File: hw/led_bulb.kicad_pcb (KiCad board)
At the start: 2 copper layers, 136 x 50 mm, 181 parts, among them P1 USB_OTG, P10 CONN_01X04, P11 CONN_01X04, P12 CONN_01X04, P13 CONN_01X04, P14 CONN_01X04, P15 CONN_01X04, P16 CONN_01X04, P17 CONN_01X04, P2 CONN_01X04, P3 CONN_01X04, P4 CONN_01X04, P5 CONN_01X04, P6 CONN_01X04, P7 CONN_01X04, P8 CONN_01X04, P9 CONN_01X04, SW1 SW_RST, SW2 SW_FLASH, U1 CP2102, U3 ESP-12E, U4 AP1117D33

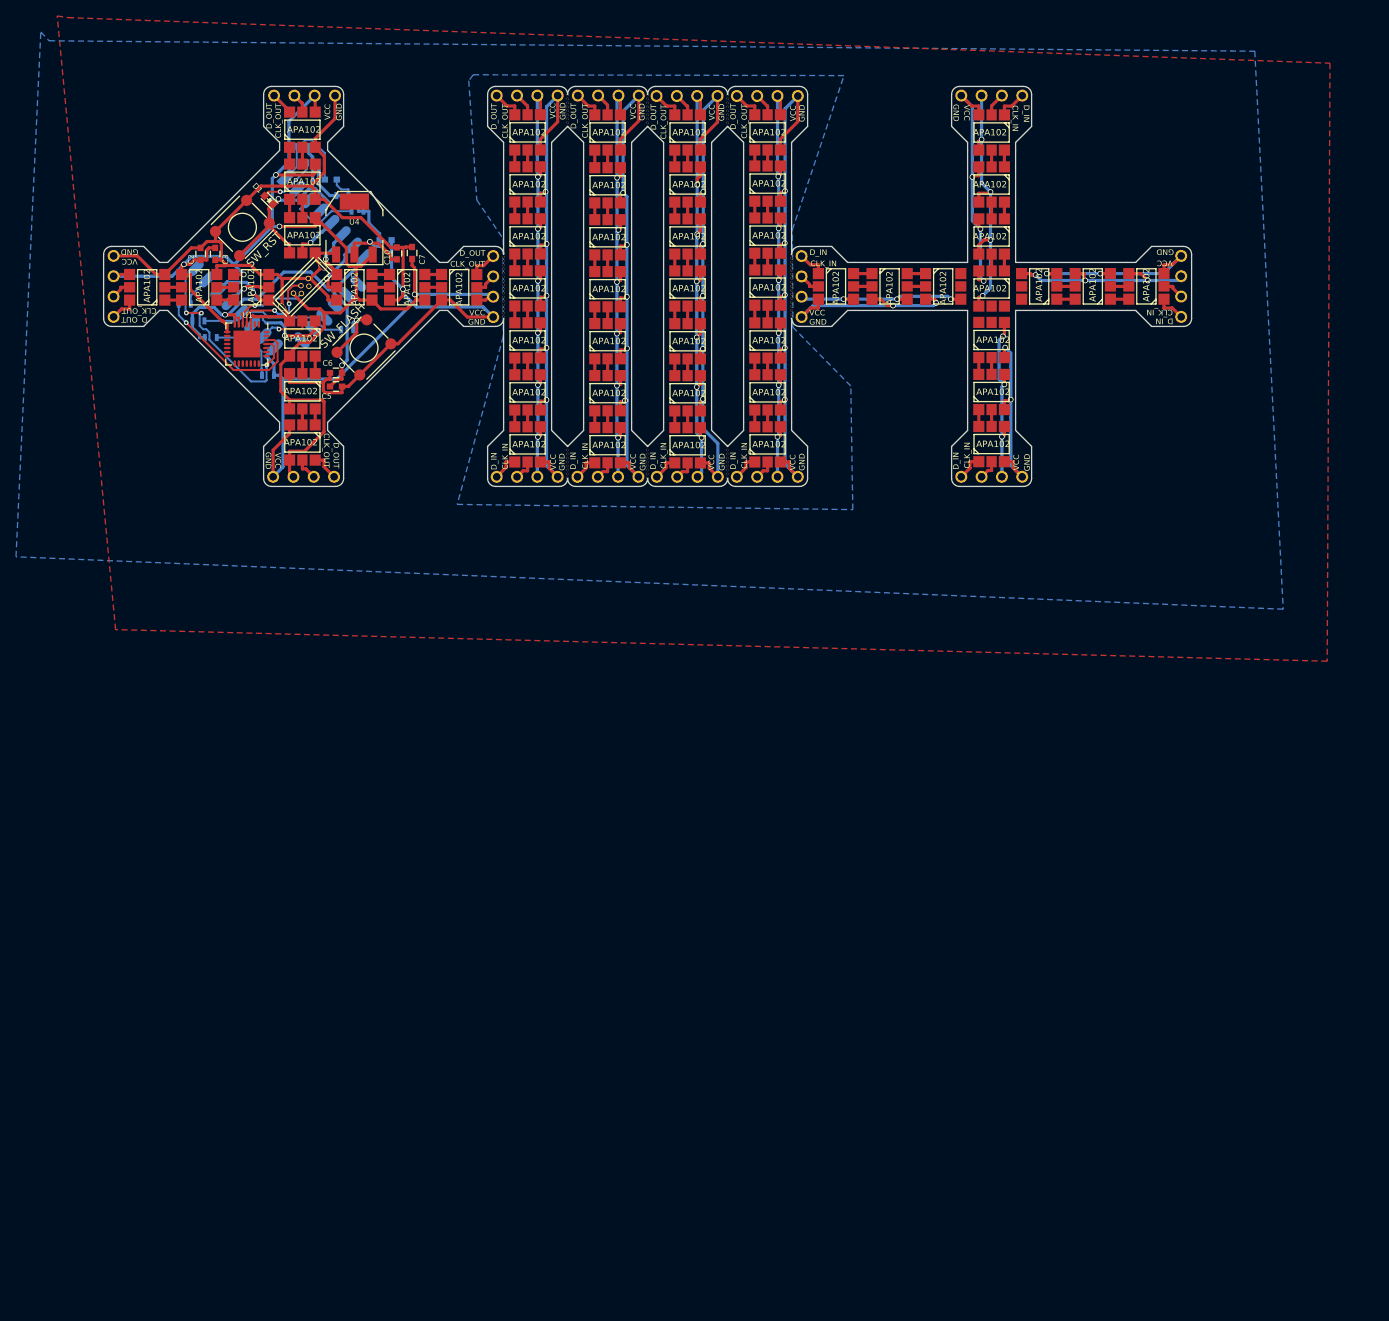
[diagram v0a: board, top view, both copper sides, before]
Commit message: Added first version of v4 hardware.
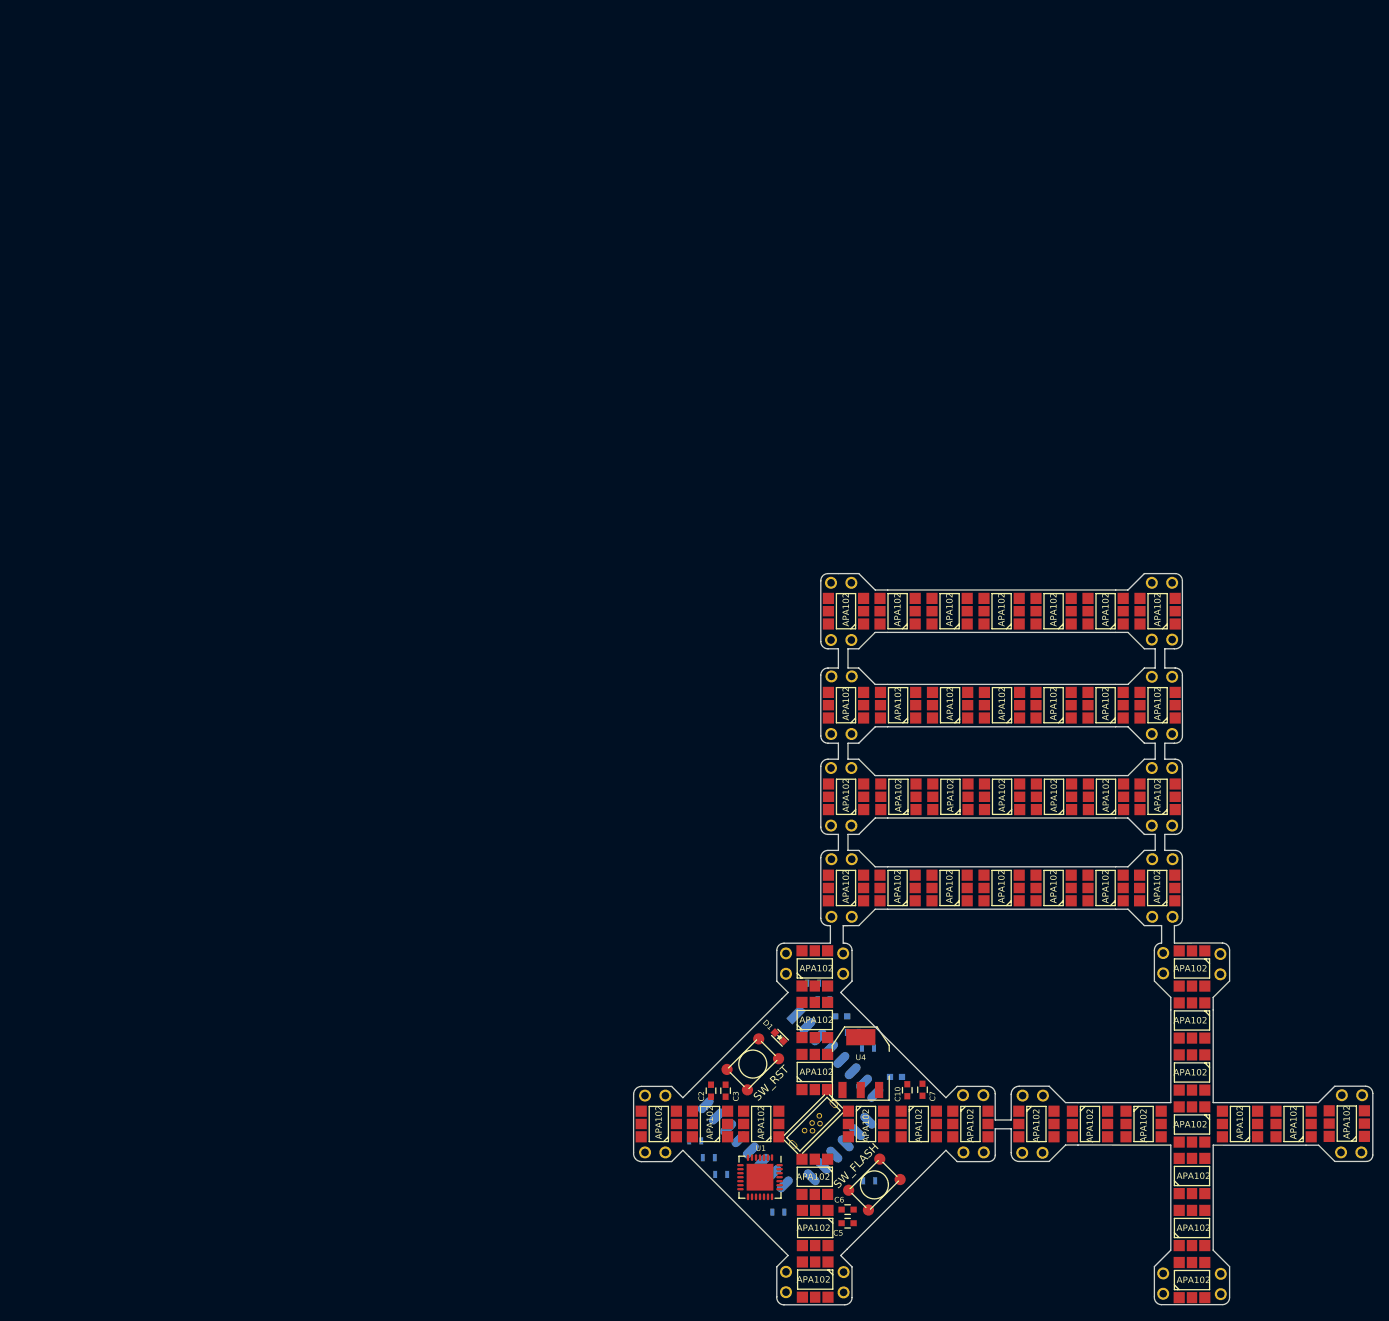
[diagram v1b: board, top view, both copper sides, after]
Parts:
- removed HOLE0 (x88): 0.3mm, footprints:0.3mm
- added P18: CONN_01X02, footprints:CONN_2.54mm_1x2_no-outline, F.Cu at (156.4, 125.6)
- added P19: CONN_01X02, footprints:CONN_2.54mm_1x2_no-outline, F.Cu at (149.2, 125.5)
- added P20: CONN_01X02, footprints:CONN_2.54mm_1x2_no-outline, F.Cu at (172.8, 149.2)
- added P21: CONN_01X02, footprints:CONN_2.54mm_1x2_no-outline, F.Cu at (172.8, 142.0)
- added P22: CONN_01X02, footprints:CONN_2.54mm_1x2_no-outline, F.Cu at (149.2, 165.6)
- added P23: CONN_01X02, footprints:CONN_2.54mm_1x2_no-outline, F.Cu at (156.4, 165.6)
- added P24: CONN_01X02, footprints:CONN_2.54mm_1x2_no-outline, F.Cu at (132.9, 142.1)
- added P25: CONN_01X02, footprints:CONN_2.54mm_1x2_no-outline, F.Cu at (132.9, 149.2)
- added P26: CONN_01X02, footprints:CONN_2.54mm_1x2_no-outline, F.Cu at (109.0, 85.1)
- added P27: CONN_01X02, footprints:CONN_2.54mm_1x2_no-outline, F.Cu at (109.0, 78.0)
- added P28: CONN_01X02, footprints:CONN_2.54mm_1x2_no-outline, F.Cu at (109.0, 96.8)
- added P29: CONN_01X02, footprints:CONN_2.54mm_1x2_no-outline, F.Cu at (109.0, 89.7)
- added P30: CONN_01X02, footprints:CONN_2.54mm_1x2_no-outline, F.Cu at (109.0, 108.3)
- added P31: CONN_01X02, footprints:CONN_2.54mm_1x2_no-outline, F.Cu at (109.0, 101.1)
- added P32: CONN_01X02, footprints:CONN_2.54mm_1x2_no-outline, F.Cu at (109.0, 119.7)
- added P33: CONN_01X02, footprints:CONN_2.54mm_1x2_no-outline, F.Cu at (109.0, 112.5)
- P10, P11, P12, P13, P14, P15, P16, P17, P2, P3, P4, P5, P6, P7, P8, P9: value CONN_01X04 -> CONN_01X02; footprint footprints:CONN_2.54mm_1x4_no-outline -> footprints:CONN_2.54mm_1x2_no-outline
- SW1, SW2: footprint footprints:switch_spst_smd_5.5mm_4.5mm -> footprints:switch_spst_smd_5mm_3.5mm
- moved P5 150.2 mm to (102.1, 165.3), turned to 90 degrees
- moved R9 124.8 mm to (112.5, 152.7)
- moved P2 124.1 mm to (102.1, 125.5), turned to 270 degrees
- moved LED9 122.9 mm to (105.7, 126.2)
- moved LED3 122.8 mm to (105.7, 152.2)
- moved LED5 122.8 mm to (105.7, 132.6)
- moved LED11 122.7 mm to (105.8, 165.1)
- moved LED7 122.7 mm to (105.8, 158.6)
- moved LED1 122.6 mm to (105.7, 139.1)
- moved P1 122.6 mm to (103.8, 149.0)
- moved LED12 122.6 mm to (86.2, 145.6)
- moved LED6 122.6 mm to (118.7, 145.6)
- moved C5 122.6 mm to (109.8, 158.0)
- moved C6 122.6 mm to (109.8, 156.3)
- moved LED2 122.6 mm to (112.1, 145.6)
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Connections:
- net DTR renamed Net-(U1-Pad28)
- net RTS renamed Net-(U1-Pad24)
- LED1 pad 1: GPIO16 -> GPIO0
- LED13 pad 3: GND -> Net-(LED13-Pad3)
- LED13 pad 4: V_USB -> Net-(LED13-Pad4)
- LED14 pad 3: GND -> Net-(LED14-Pad3)
- LED14 pad 4: V_USB -> Net-(LED14-Pad4)
- LED15 pad 3: GND -> Net-(LED15-Pad3)
- LED15 pad 4: V_USB -> Net-(LED15-Pad4)
- LED16 pad 3: GND -> Net-(LED16-Pad3)
- LED16 pad 4: V_USB -> Net-(LED16-Pad4)
- LED17 pad 3: GND -> Net-(LED13-Pad3)
- LED17 pad 4: V_USB -> Net-(LED13-Pad4)
- LED18 pad 3: GND -> Net-(LED14-Pad3)
- LED18 pad 4: V_USB -> Net-(LED14-Pad4)
- LED19 pad 3: GND -> Net-(LED15-Pad3)
- LED19 pad 4: V_USB -> Net-(LED15-Pad4)
- LED20 pad 3: GND -> Net-(LED16-Pad3)
- LED20 pad 4: V_USB -> Net-(LED16-Pad4)
- LED21 pad 3: GND -> Net-(LED13-Pad3)
- LED21 pad 4: V_USB -> Net-(LED13-Pad4)
- LED22 pad 3: GND -> Net-(LED14-Pad3)
- LED22 pad 4: V_USB -> Net-(LED14-Pad4)
- LED23 pad 3: GND -> Net-(LED15-Pad3)
- LED23 pad 4: V_USB -> Net-(LED15-Pad4)
- LED24 pad 3: GND -> Net-(LED16-Pad3)
- LED24 pad 4: V_USB -> Net-(LED16-Pad4)
- LED25 pad 3: GND -> Net-(LED13-Pad3)
- LED25 pad 4: V_USB -> Net-(LED13-Pad4)
- LED26 pad 3: GND -> Net-(LED14-Pad3)
- LED26 pad 4: V_USB -> Net-(LED14-Pad4)
- LED27 pad 3: GND -> Net-(LED15-Pad3)
- LED27 pad 4: V_USB -> Net-(LED15-Pad4)
- LED28 pad 3: GND -> Net-(LED16-Pad3)
- LED28 pad 4: V_USB -> Net-(LED16-Pad4)
- LED29 pad 3: GND -> Net-(LED13-Pad3)
- LED29 pad 4: V_USB -> Net-(LED13-Pad4)
- LED30 pad 3: GND -> Net-(LED14-Pad3)
- LED30 pad 4: V_USB -> Net-(LED14-Pad4)
- LED31 pad 3: GND -> Net-(LED15-Pad3)
- LED31 pad 4: V_USB -> Net-(LED15-Pad4)
- LED32 pad 3: GND -> Net-(LED16-Pad3)
- LED32 pad 4: V_USB -> Net-(LED16-Pad4)
- LED33 pad 3: GND -> Net-(LED13-Pad3)
- LED33 pad 4: V_USB -> Net-(LED13-Pad4)
- LED34 pad 3: GND -> Net-(LED14-Pad3)
- LED34 pad 4: V_USB -> Net-(LED14-Pad4)
- LED35 pad 3: GND -> Net-(LED15-Pad3)
- LED35 pad 4: V_USB -> Net-(LED15-Pad4)
- LED36 pad 3: GND -> Net-(LED16-Pad3)
- LED36 pad 4: V_USB -> Net-(LED16-Pad4)
- LED37 pad 3: GND -> Net-(LED13-Pad3)
- LED37 pad 4: V_USB -> Net-(LED13-Pad4)
- LED38 pad 3: GND -> Net-(LED14-Pad3)
- LED38 pad 4: V_USB -> Net-(LED14-Pad4)
- LED39 pad 3: GND -> Net-(LED15-Pad3)
- LED39 pad 4: V_USB -> Net-(LED15-Pad4)
- LED40 pad 3: GND -> Net-(LED16-Pad3)
- LED40 pad 4: V_USB -> Net-(LED16-Pad4)
- LED41 pad 3: GND -> Net-(LED41-Pad3)
- LED41 pad 4: V_USB -> Net-(LED41-Pad4)
- LED42 pad 3: GND -> Net-(LED42-Pad3)
- LED42 pad 4: V_USB -> Net-(LED42-Pad4)
- LED43 pad 3: GND -> Net-(LED43-Pad3)
- LED43 pad 4: V_USB -> Net-(LED43-Pad4)
- LED44 pad 3: GND -> Net-(LED44-Pad3)
- LED44 pad 4: V_USB -> Net-(LED44-Pad4)
- LED45 pad 3: GND -> Net-(LED42-Pad3)
- LED45 pad 4: V_USB -> Net-(LED42-Pad4)
- LED46 pad 3: GND -> Net-(LED41-Pad3)
- LED46 pad 4: V_USB -> Net-(LED41-Pad4)
- LED47 pad 3: GND -> Net-(LED43-Pad3)
- LED47 pad 4: V_USB -> Net-(LED43-Pad4)
- LED48 pad 3: GND -> Net-(LED44-Pad3)
- LED48 pad 4: V_USB -> Net-(LED44-Pad4)
- LED49 pad 3: GND -> Net-(LED42-Pad3)
- LED49 pad 4: V_USB -> Net-(LED42-Pad4)
- LED50 pad 3: GND -> Net-(LED41-Pad3)
- LED50 pad 4: V_USB -> Net-(LED41-Pad4)
- LED51 pad 3: GND -> Net-(LED43-Pad3)
- LED51 pad 4: V_USB -> Net-(LED43-Pad4)
- LED52 pad 3: GND -> Net-(LED44-Pad3)
- LED52 pad 4: V_USB -> Net-(LED44-Pad4)
- LED53 pad 3: GND -> Net-(LED41-Pad3)
- LED53 pad 4: V_USB -> Net-(LED41-Pad4)
- P10 pad 1: Net-(LED37-Pad6) -> Net-(LED13-Pad2)
- P10 pad 2: Net-(LED37-Pad5) -> Net-(LED13-Pad1)
- P11 pad 1: Net-(LED38-Pad6) -> Net-(LED13-Pad3)
- P11 pad 2: Net-(LED38-Pad5) -> Net-(LED13-Pad4)
- P12 pad 1: Net-(LED39-Pad6) -> Net-(LED14-Pad2)
- P12 pad 2: Net-(LED39-Pad5) -> Net-(LED14-Pad1)
- P13 pad 1: Net-(LED40-Pad6) -> Net-(LED14-Pad3)
- P13 pad 2: Net-(LED40-Pad5) -> Net-(LED14-Pad4)
- P14 pad 1: GND -> Net-(LED15-Pad2)
- P14 pad 2: V_USB -> Net-(LED15-Pad1)
- P15 pad 1: GND -> Net-(LED15-Pad3)
- P15 pad 2: V_USB -> Net-(LED15-Pad4)
- P16 pad 1: GND -> Net-(LED16-Pad2)
- P16 pad 2: V_USB -> Net-(LED16-Pad1)
- P17 pad 1: GND -> Net-(LED16-Pad3)
- P17 pad 2: V_USB -> Net-(LED16-Pad4)
- P3 pad 1: Net-(LED10-Pad6) -> V_USB
- P3 pad 2: Net-(LED10-Pad5) -> GND
- P4 pad 1: Net-(LED11-Pad6) -> Net-(LED10-Pad6)
- P4 pad 2: Net-(LED11-Pad5) -> Net-(LED10-Pad5)
- P5 pad 1: Net-(LED12-Pad6) -> V_USB
- P5 pad 2: Net-(LED12-Pad5) -> GND
- P6 pad 1: GND -> Net-(LED11-Pad6)
- P6 pad 2: V_USB -> Net-(LED11-Pad5)
- P7 pad 1: GND -> V_USB
- P7 pad 2: V_USB -> GND
- P8 pad 1: GND -> Net-(LED12-Pad6)
- P8 pad 2: V_USB -> Net-(LED12-Pad5)
- P9 pad 1: GND -> V_USB
- P9 pad 2: V_USB -> GND
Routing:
- net GND: track 595.8 -> 0.00 mm, vias 30 -> 0
- net V_USB: track 508.1 -> 0.00 mm, vias 42 -> 0
- net V_3.3: track 76.2 -> 0.00 mm, vias 3 -> 0
- net GPIO16: track 28.6 -> 0.00 mm, vias 1 -> 0
- net TX: track 27.7 -> 0.00 mm, vias 3 -> 0
- net Net-(R8-Pad1): track 21.2 -> 0.00 mm, vias 1 -> 0
- net GPIO0: track 18.6 -> 0.00 mm
- net GPIO2: track 16.8 -> 0.00 mm, vias 1 -> 0
- net nRST: track 12.5 -> 0.00 mm
- net GPIO15: track 12.2 -> 0.00 mm, vias 1 -> 0
- net USB_D+: track 11.5 -> 0.00 mm, vias 2 -> 0
- net USB_D-: track 9.94 -> 0.00 mm, vias 1 -> 0
- net EN: track 9.22 -> 0.00 mm
- net LED4_DATA: track 8.03 -> 0.00 mm, vias 1 -> 0
- net LED2_CLK: track 7.80 -> 0.00 mm, vias 1 -> 0
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- removed copper zone on B.Cu, net GND
- removed copper zone on B.Cu, net V_USB
- removed copper zone on F.Cu, net V_USB
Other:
- board size 136 x 50 mm -> 92.4 x 91.4 mm
- board text added: "esp8266_apa102_bulb v4"
- board text removed: "CLK_IN"
- board text removed: "CLK_OUT"
- board text removed: "D_IN"
- board text removed: "D_OUT"
- board text removed: "GND"
- board text removed: "VCC"
- board text removed: "esp8266_apa102_bulb v3.0"
